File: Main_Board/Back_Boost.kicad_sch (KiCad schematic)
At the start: 8 parts, among them U3 TPS63031DSK

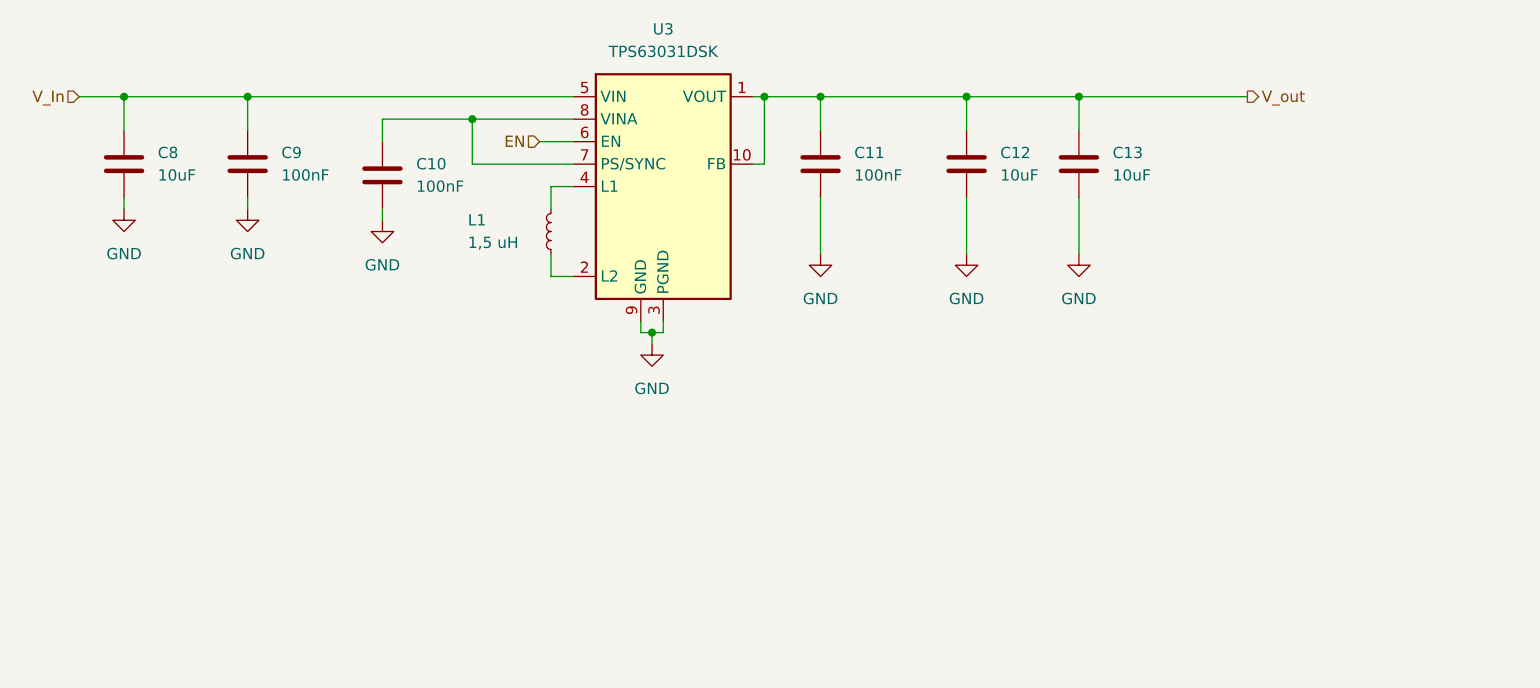
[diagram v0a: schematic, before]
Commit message: Fix schematic readibility
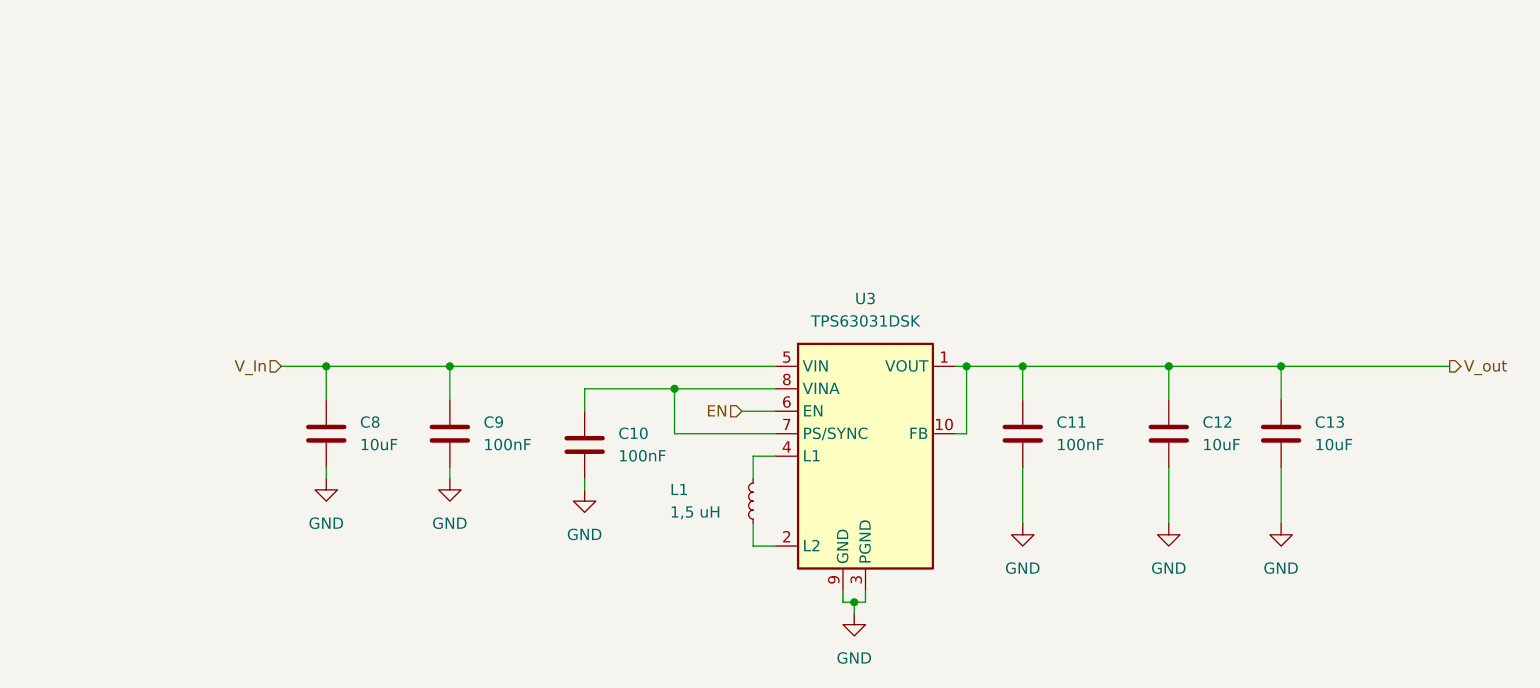
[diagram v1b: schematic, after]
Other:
- moved on the sheet: C10, C11, C12, C13, C8, C9, L1, U3
